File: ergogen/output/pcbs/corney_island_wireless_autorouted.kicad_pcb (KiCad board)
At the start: 2 copper layers, 133.8 x 91.7 mm, 68 parts

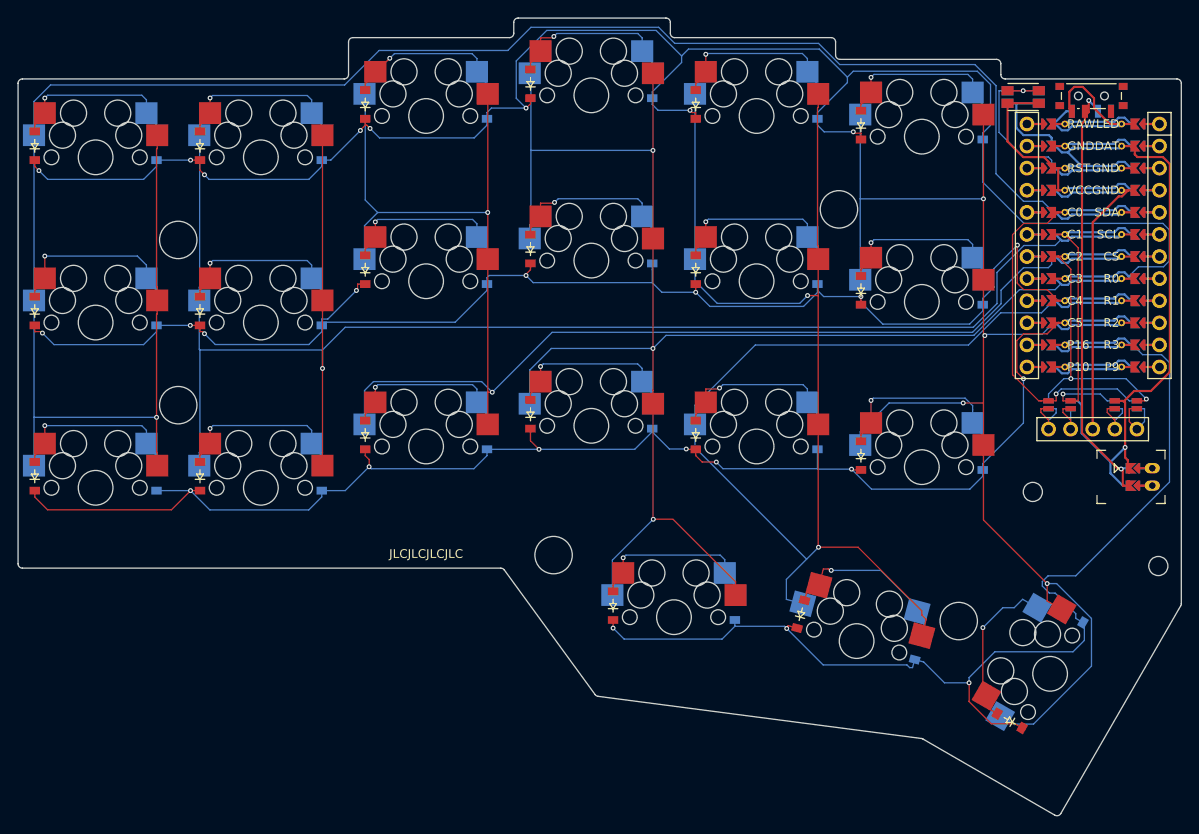
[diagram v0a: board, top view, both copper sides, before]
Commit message: Update assets
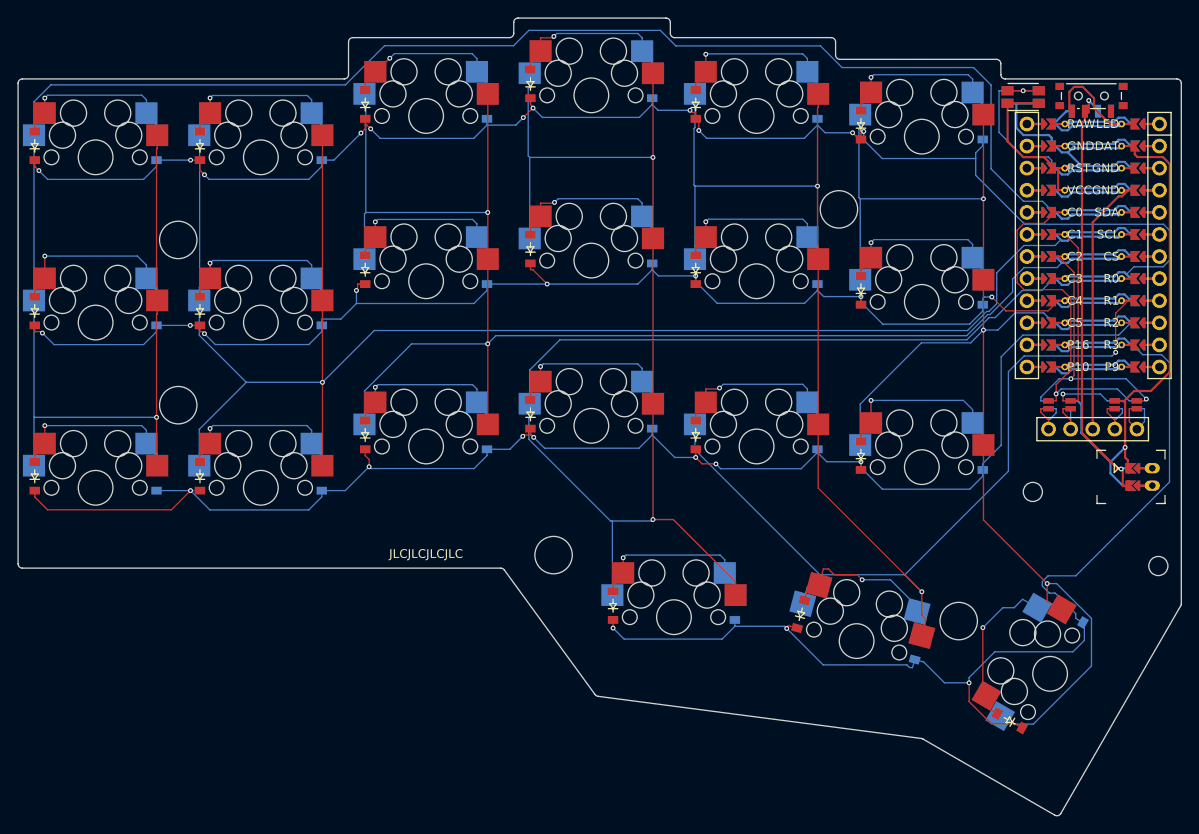
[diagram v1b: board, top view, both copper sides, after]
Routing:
- net R0: track 215.1 -> 178.4 mm, vias 8 -> 11
- net C3: track 188.3 -> 208.1 mm, vias 3 -> 2
- net R1: track 165.9 -> 154.4 mm
- net R2: track 168.0 -> 175.4 mm
- net C5: track 155.7 -> 161.9 mm, vias 4 -> 3
- net C4: track 196.2 -> 198.8 mm, vias 2 -> 3
- net SDA: track 49.7 -> 51.8 mm
- net CS: track 39.7 -> 41.6 mm
- net C1: track 194.7 -> 193.2 mm
- net C2: track 173.3 -> 172.3 mm
- net C0: track 239.8 -> 239.2 mm
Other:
- outline, holes or cut-outs redrawn
- net class Default added: clearance 0.2, trace_width 0.25, via_dia 0.8, via_drill 0.4

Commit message: Update assets
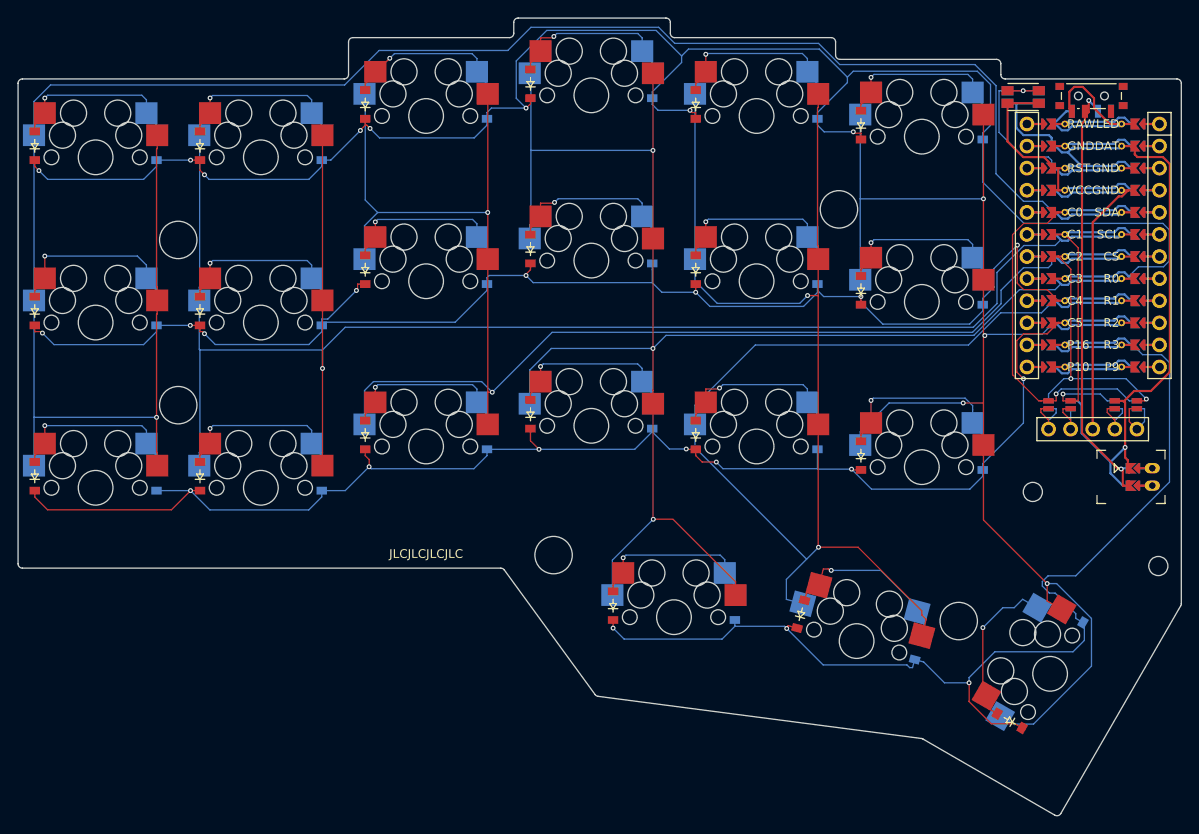
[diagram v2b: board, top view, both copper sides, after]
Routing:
- net R0: track 178.4 -> 215.1 mm, vias 11 -> 8
- net C3: track 208.1 -> 188.3 mm, vias 2 -> 3
- net R1: track 154.4 -> 165.9 mm
- net R2: track 175.4 -> 168.0 mm
- net C5: track 161.9 -> 155.7 mm, vias 3 -> 4
- net C4: track 198.8 -> 196.2 mm, vias 3 -> 2
- net SDA: track 51.8 -> 49.7 mm
- net CS: track 41.6 -> 39.7 mm
- net C1: track 193.2 -> 194.7 mm
- net C2: track 172.3 -> 173.3 mm
- net C0: track 239.2 -> 239.8 mm
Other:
- outline, holes or cut-outs redrawn
- net class Default removed
